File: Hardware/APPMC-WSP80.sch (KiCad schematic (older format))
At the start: 83 parts, among them J1 + 30V max, J10 STLINK-V3, J101 ADC_C, J102 ADC_D, J14 VDD, J15 PWM, J16 ADC_B, J17 3.0V, J18 1.5V, J2 VOut, J20 ADC_A, J23 GND, J4 Jumper-2B-Open, J6 STLINK-V2, J9 Waveshare 18179, M4 Logo_Open_Hardware_Small, Q1 SI2343CDS-T1-GE3, Q2 ZXMP4A16GTA, Q3 ZXMP4A16GTA, Q4 BSS123, SW1 RESET, U1 INA823, U101 OPA320, U2 3.3V, U3 REF2030, U5 STM32G0B1CEUx, U6 24CW640T-I/OT

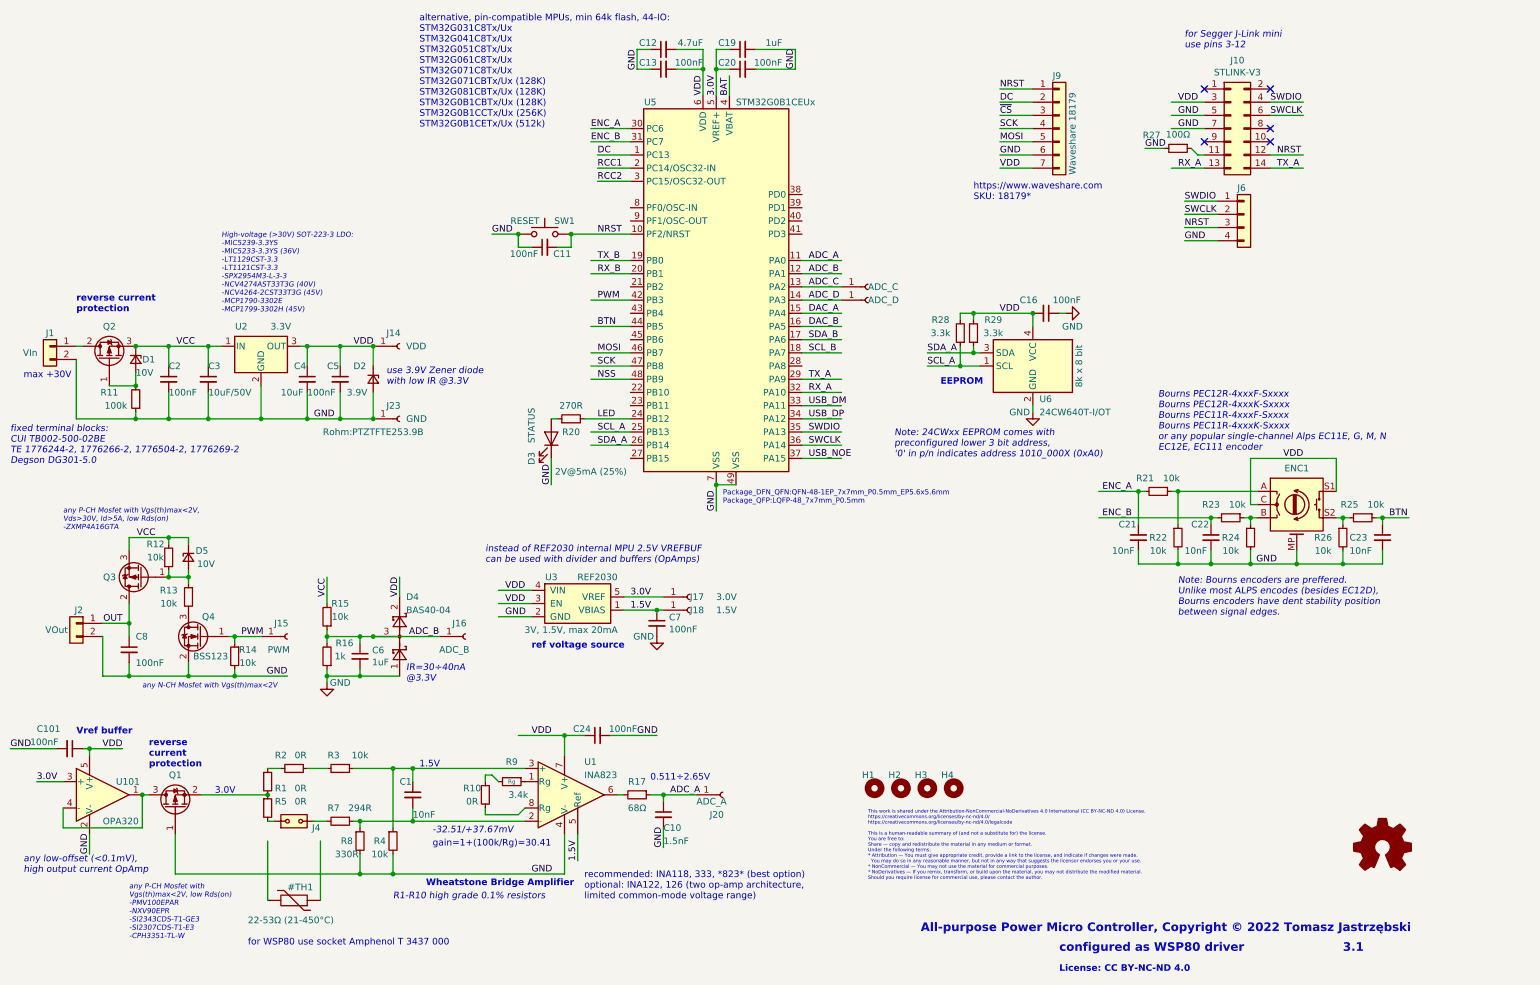
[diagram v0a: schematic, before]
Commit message: update
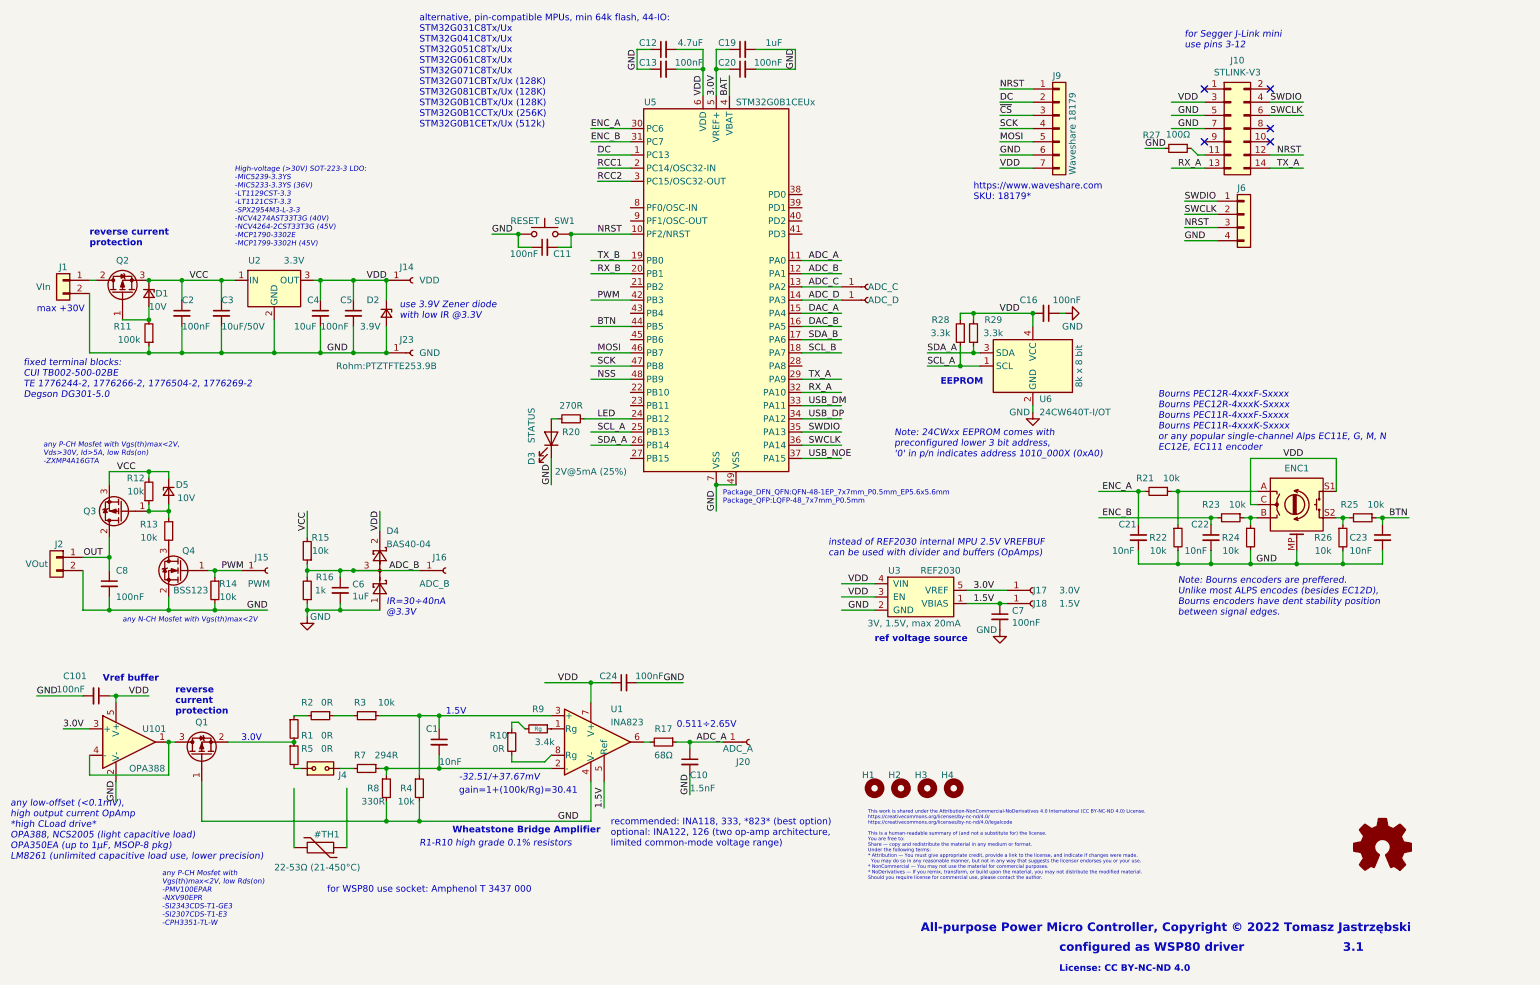
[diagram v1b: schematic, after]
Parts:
- U101: value OPA320 -> OPA388
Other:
- note added: "any low-offset (<0.1mV),\nhigh output current OpAmp\n*high CLoad drive*\nOPA388, NCS2005 (light capacitive load)\nOPA350EA (up to 1µF, MSOP-8 pkg)\nLM8261 (unlimited capacitive load use, lower precision)"
- note added: "for WSP80 use socket: Amphenol T 3437 000"
- note removed: "any low-offset (<0.1mV),\nhigh output current OpAmp"
- note removed: "for WSP80 use socket Amphenol T 3437 000"
- moved on the sheet: C1, C10, C101, C2, C24, C3, C4, C5, C6, C7, C8, D1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
